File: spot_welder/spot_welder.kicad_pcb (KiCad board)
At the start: 2 copper layers, 93.7 x 117.2 mm, 95 parts, among them J1 Trigger, J2 Conn_SWD, J3 External_Power, Q1 NX3020NAKW, Q2 HY4903B6, Q3 HY4903B6, Q4 HY4903B6, Q5 HY4903B6, Q6 HY4903B6, Q7 HY4903B6, U1 STM32F103C8Tx, U2 SN74LVC1G123DCT, U3 LM2575-ADJ, U4 IRS44273LTRPBF, U5 AMS1117-3.3, U6 RC1602A

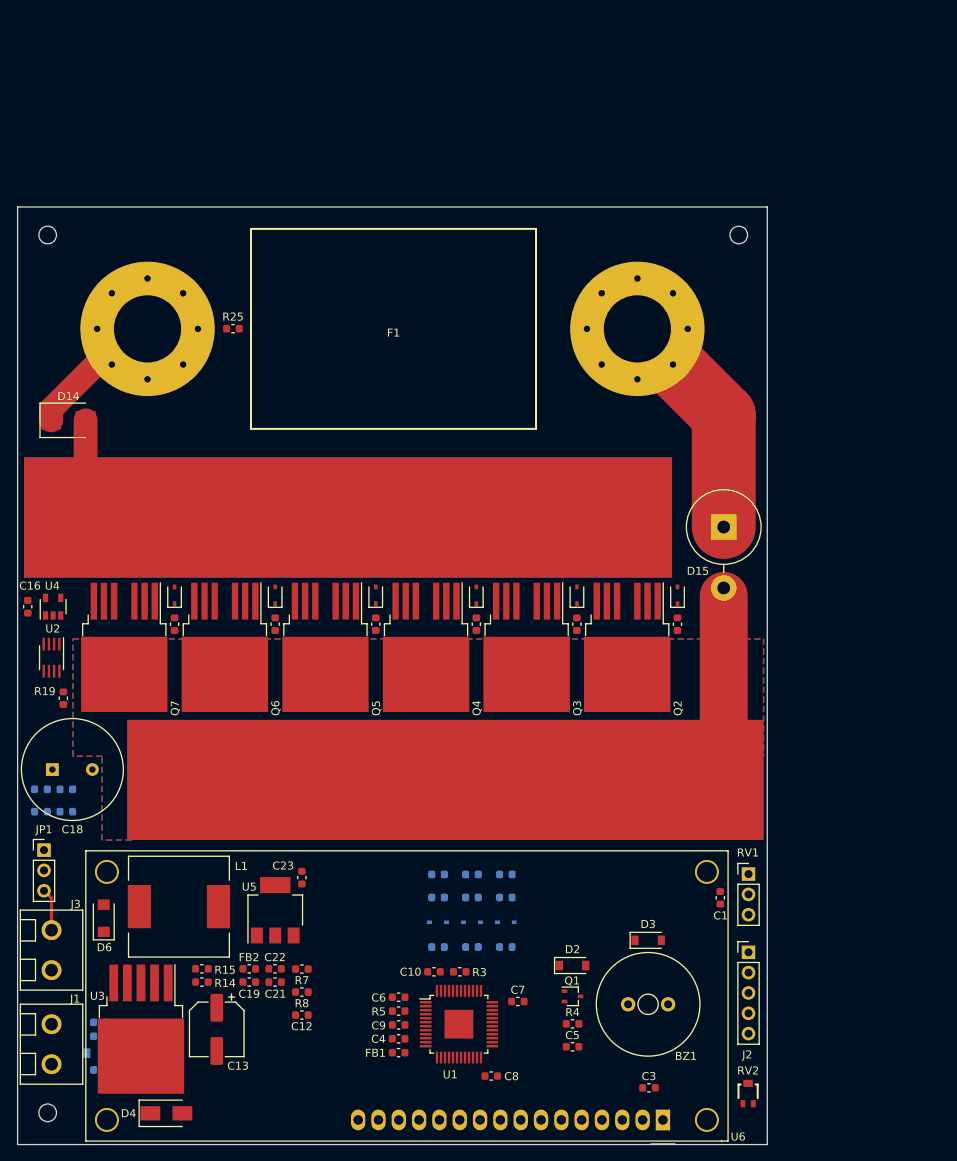
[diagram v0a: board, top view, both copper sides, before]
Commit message: 1
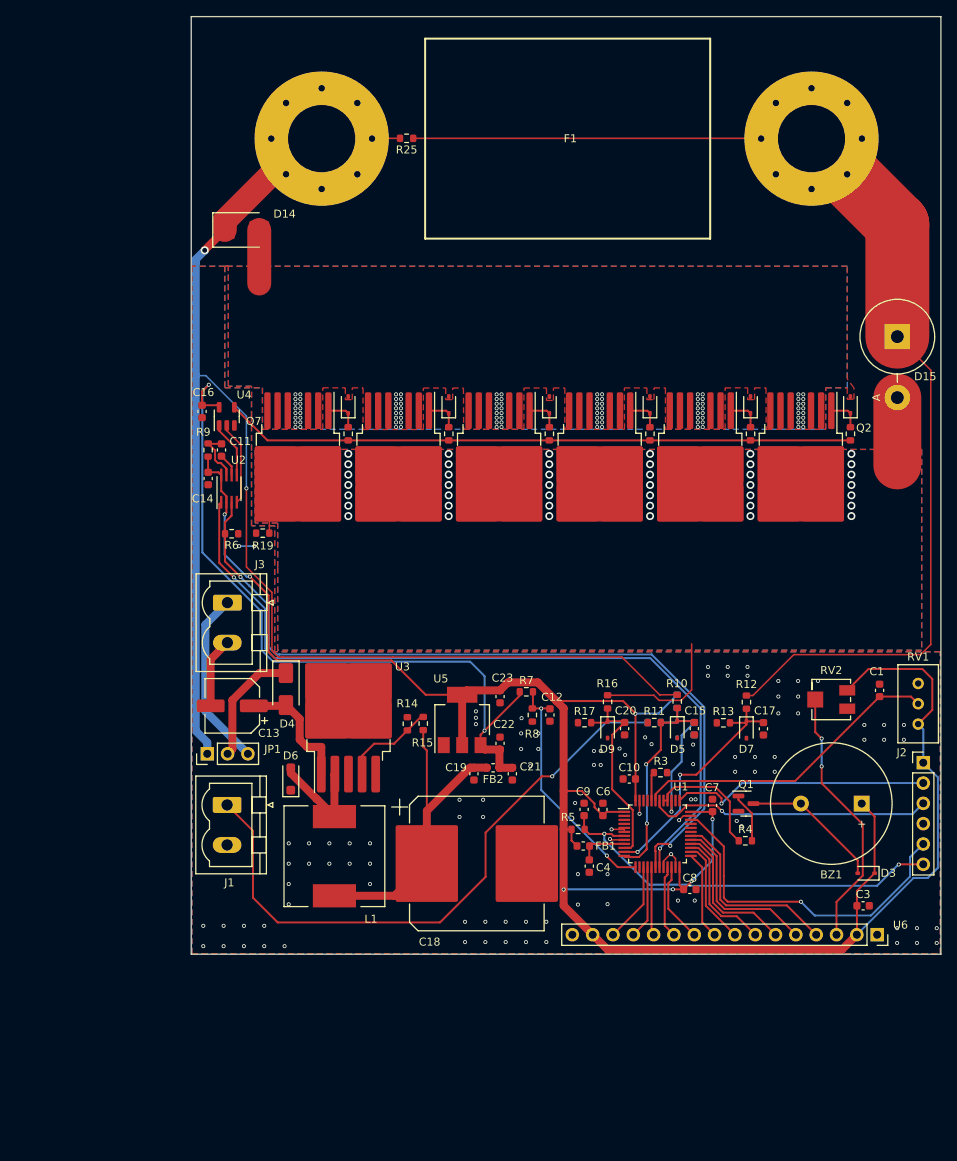
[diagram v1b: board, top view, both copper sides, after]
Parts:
- removed C5: 10nF, Capacitor_SMD:C_0603_1608Metric
- removed D2: 1N4148, Diode_SMD:D_SOD-123
- removed the REF** at (99.2, 122.4) (x2)
- removed the REF** at (89.6, 89.6) (x2)
- removed the REF** at (138.4, 54.3)
- removed the REF** at (52.0, 54.3)
- removed the REF** at (52.0, 164.0)
- added REF**: Logo, KIGIT_Footprints:Logo, B.Cu at (116.9, 34.8)
- BZ1: value PS1240P02BT -> SFN-1407PA7.6; footprint spot_welder:BUZ-TH_BD12.5-P5.00-D0.9 -> Buzzer_Beeper:Buzzer_15x7.5RM7.6
- C11, C14, C15, C17, C20, D5, D7, D9, R10, R11, R12, R13, R16, R17, R6, R9: moved to F.Cu
- C18: value 16V 2200uF -> 16V 2200u; footprint Capacitor_THT:C_Radial_D12.5mm_H20.0mm_P5.00mm -> Capacitor_SMD:CP_Elec_16x17.5
- C3, C4: value 50V 1uF -> 1uF
- D1: value BZT52C4V7 -> MM3Z4V7; footprint Diode_SMD:D_SOD-123 -> Diode_SMD:D_SOD-323
- D15: value nb -> nc(BZW50-68)
- D3: value 1N4148 -> nc(1N4148WS); footprint Diode_SMD:D_SOD-123 -> Diode_SMD:D_SOD-323
- D6: footprint spot_welder:D_SOD-123FL -> Diode_SMD:D_SOD-123F
- J1, J3: footprint spot_welder:CONN-5.0-2P -> Connector_Phoenix_MSTB:PhoenixContact_MSTBVA_2,5_2-G_1x02_P5.00mm_Vertical
- J2: footprint Connector_PinHeader_2.54mm:PinHeader_1x05_P2.54mm_Vertical -> Connector_PinHeader_2.54mm:PinHeader_1x06_P2.54mm_Vertical
- Q1: value NX3020NAKW -> 2N4401; footprint Package_TO_SOT_SMD:SOT-323_SC-70 -> Package_TO_SOT_SMD:SOT-23
- R4: value 220k -> 1k
- RV1: footprint Connector_PinHeader_2.54mm:PinHeader_1x03_P2.54mm_Vertical -> Potentiometer_THT:Potentiometer_Bourns_3386C_Horizontal
- RV2: footprint spot_welder:EVM2GSX80B14 -> Potentiometer_SMD:Potentiometer_Bourns_3214J_Horizontal
- U1: value STM32F103C8Tx -> STM32F103C8T6; footprint Package_QFP:LQFP-48-1EP_7x7mm_P0.5mm_EP3.6x3.6mm -> Package_QFP:LQFP-48_7x7mm_P0.5mm
- U6: value RC1602A -> HS1602A; footprint spot_welder:RC1602A -> Connector_PinSocket_2.54mm:PinSocket_1x16_P2.54mm_Vertical
- moved C2 85.7 mm to (132.8, 116.0), turned to -90 degrees
- moved D1 82.7 mm to (130.7, 116.1), turned to -90 degrees
- moved R2 82.6 mm to (130.7, 112.6), turned to -90 degrees
- moved R1 79.6 mm to (127.8, 115.2)
- moved D4 55.1 mm to (81.8, 111.1), turned to -90 degrees
- moved C11 50.5 mm to (73.7, 81.2), turned to -90 degrees
- moved RV2 50.2 mm to (150.0, 112.4)
- moved C18 49.5 mm to (105.7, 132.9), turned to 0 degrees
- moved J3 48.7 mm to (74.5, 100.3)
- moved C12 48.7 mm to (114.8, 114.3), turned to -90 degrees
- moved U3 47.3 mm to (89.6, 114.0), turned to 90 degrees
- moved R9 47.3 mm to (72.1, 81.2), turned to -90 degrees
- moved C17 45.5 mm to (141.5, 116.0), turned to -90 degrees
- moved R8 45.0 mm to (112.6, 114.3), turned to 90 degrees
- moved R7 44.6 mm to (111.9, 111.4)
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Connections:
- net /SWDCLK renamed /RXD_SWDCLK
- BZ1 pad 2: Net-(BZ1-Pad2) -> Net-(BZ1-+)
- C14 pad 1: +3V3 -> VBAT-
- C14 pad 2: VBAT- -> +3V3
- C16 pad 1: +3V3 -> +10V
- D3 pad 2: Net-(BZ1-Pad2) -> Net-(BZ1-+)
- J2 pad 3: VBAT- -> /TXD
- J2 pad 4: /SWDIO -> VBAT-
- J2 pad 5: /NRST -> /SWDIO
- Q1 pad 1: Net-(BZ1-Pad2) -> Net-(Q1-B)
- Q1 pad 2: Net-(C5-Pad1) -> VBAT-
- Q1 pad 3: VBAT- -> Net-(BZ1-+)
- R4 pad 1: Net-(C5-Pad1) -> /BUZZER
- R4 pad 2: VBAT- -> Net-(Q1-B)
- U1 pad 14: /DIAL -> unconnected-(U1-PA4-Pad14)
- U1 pad 15: /LED_D0 -> /LED_D7
- U1 pad 16: /LED_D1 -> /LED_D6
- U1 pad 17: /LED_D2 -> /LED_D5
- U1 pad 18: /LED_E -> /SW_OFF
- U1 pad 19: /LED_RW -> /SW_ON
- U1 pad 2: Net-(U1-Pad2) -> unconnected-(U1-PC13-Pad2)
- U1 pad 20: Net-(U1-Pad20) -> VBAT-
- U1 pad 21: Net-(U1-Pad21) -> /LED_D4
- U1 pad 22: Net-(U1-Pad22) -> /LED_D3
- U1 pad 25: Net-(U1-Pad25) -> /LED_D2
- U1 pad 26: Net-(U1-Pad26) -> /LED_D1
- U1 pad 27: Net-(U1-Pad27) -> /LED_D0
- U1 pad 28: Net-(U1-Pad28) -> /LED_E
- U1 pad 29: /LED_D3 -> /LED_RW
- U1 pad 3: Net-(U1-Pad3) -> unconnected-(U1-PC14-Pad3)
- U1 pad 30: /LED_D4 -> /LED_RS
- U1 pad 31: /LED_D5 -> unconnected-(U1-PA10-Pad31)
- U1 pad 32: /LED_D6 -> unconnected-(U1-PA11-Pad32)
- U1 pad 33: /LED_D7 -> unconnected-(U1-PA12-Pad33)
- U1 pad 38: Net-(U1-Pad38) -> unconnected-(U1-PA15-Pad38)
- U1 pad 39: Net-(U1-Pad39) -> /TRIGGER
- U1 pad 4: Net-(U1-Pad4) -> unconnected-(U1-PC15-Pad4)
- U1 pad 40: Net-(U1-Pad40) -> /BUZZER
- U1 pad 41: /LED_RS -> /BUZZER
- U1 pad 42: /SW_OFF -> /TXD
- U1 pad 43: /SW_ON -> /DIAL
- U1 pad 45: /TRIGGER -> unconnected-(U1-PB8-Pad45)
- U1 pad 46: /BUZZER -> unconnected-(U1-PB9-Pad46)
- U1 pad 5: Net-(U1-Pad5) -> VBAT-
- U1 pad 6: Net-(U1-Pad6) -> VBAT-
- U4 pad 3: Net-(U4-Pad3) -> unconnected-(U4-OUT-Pad3)
- U4 pad 5: +3V3 -> +10V
- U6 pad 15: VBAT- -> +3V3
- U6 pad 16: +3V3 -> VBAT-
- U6 pad 4: /LED_E -> /LED_RS
- U6 pad 6: /LED_RS -> /LED_E
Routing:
- net +3V3: track 0.00 -> 282.1 mm, vias 0 -> 7
- net VBAT+: track 9.28 -> 187.1 mm, vias 0 -> 2
- net OUT+: track 22.9 -> 144.9 mm
- net /SW_OFF: track 0.00 -> 102.2 mm, vias 0 -> 2
- net /SW_ON: track 0.00 -> 100.4 mm, vias 0 -> 2
- net +10V: track 0.00 -> 93.4 mm, vias 0 -> 2
- net Net-(R18-Pad1): track 0.00 -> 78.7 mm
- net Net-(J1-Pin_1): track 0.00 -> 77.2 mm, vias 0 -> 1
- net /NRST: track 0.00 -> 51.3 mm, vias 0 -> 2
- net /SWDIO: track 0.00 -> 42.9 mm, vias 0 -> 1
- net Net-(C18-Pad1): track 0.00 -> 39.8 mm
- net /DIAL: track 0.00 -> 39.1 mm
- net /TXD: track 0.00 -> 35.8 mm, vias 0 -> 1
- net VBAT-: track 4.28 -> 39.2 mm, vias 0 -> 200
- net Net-(U6-VO): track 0.00 -> 33.2 mm, vias 0 -> 2
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- added copper zone on B.Cu, net VBAT-
- added copper zone on F.Cu, net VBAT-
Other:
- rule pad_to_mask_clearance: 0.051 -> 0.038
- rule solder_mask_min_width: 0.25 -> 0.1
